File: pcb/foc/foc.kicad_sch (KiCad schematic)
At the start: 38 parts, among them J6 TB_MOTOR, J7 PH_2.0, Q4 BTN8982TA, Q5 BTN8982TA, Q6 BTN8982TA, U7 INA240A2PW, U8 INA240A2PW

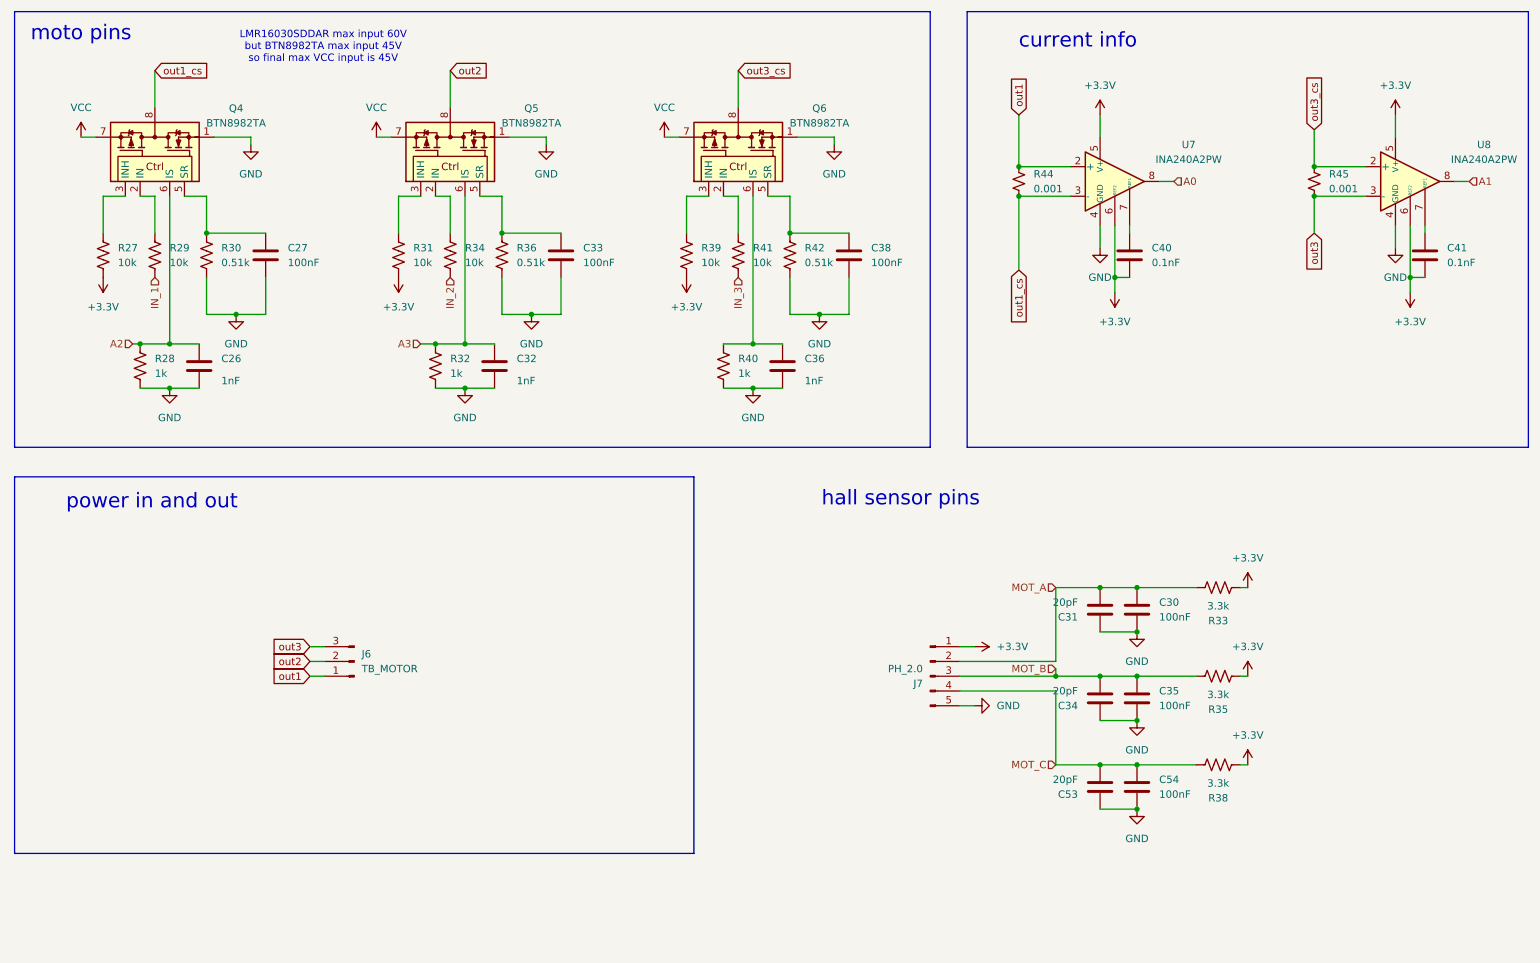
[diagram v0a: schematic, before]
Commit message: feat: update
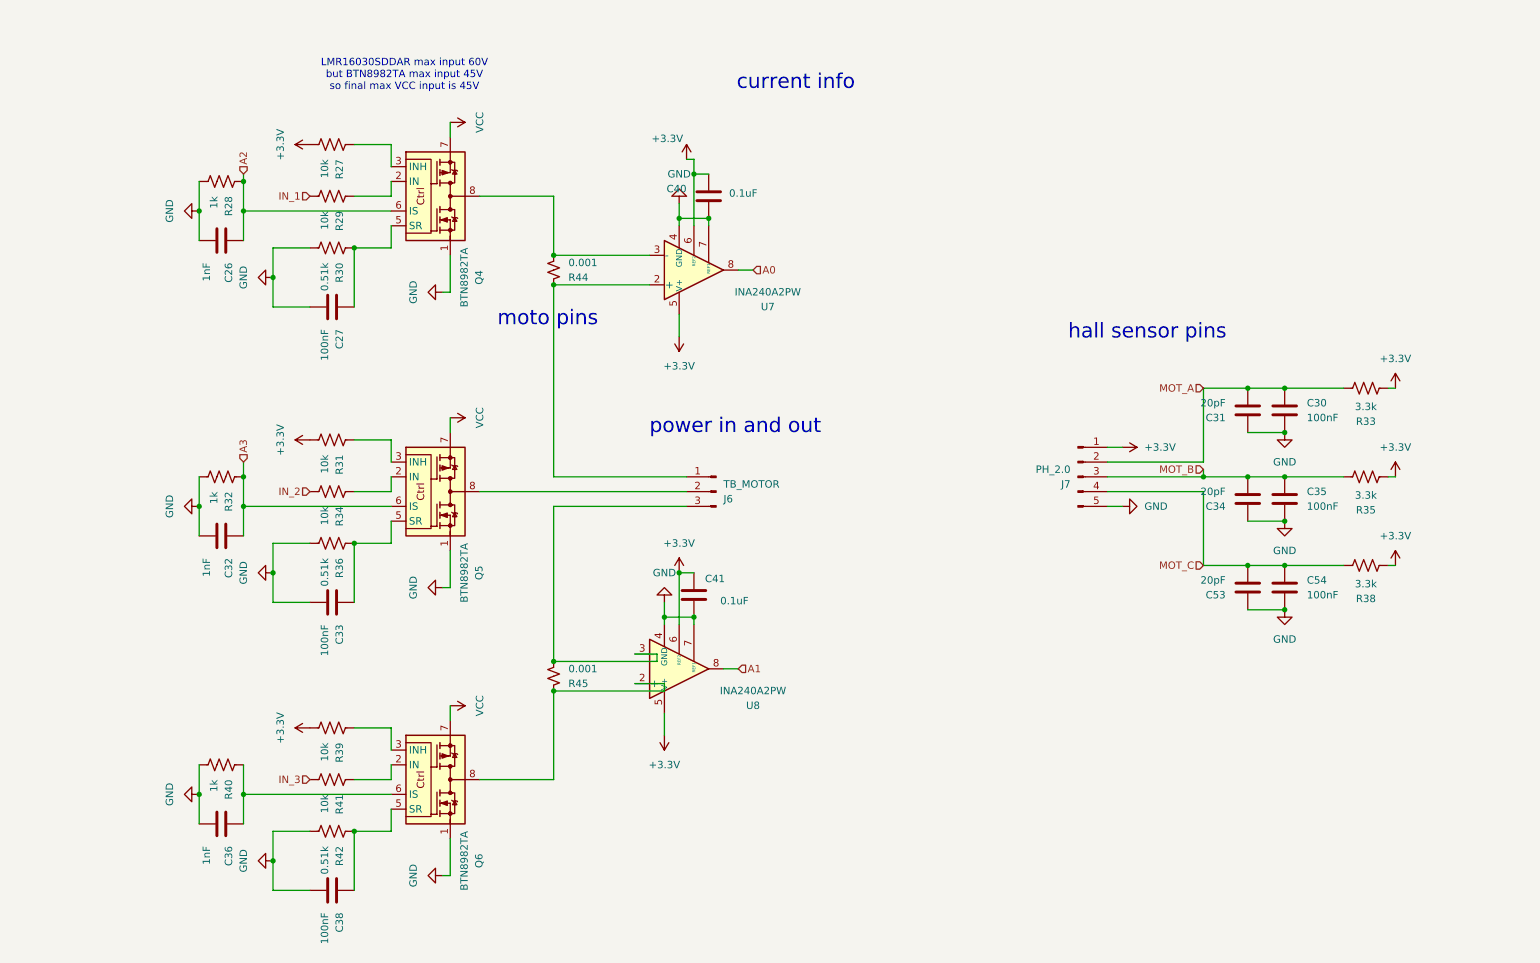
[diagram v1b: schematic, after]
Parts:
- C40, C41: value 0.1nF -> 0.1uF
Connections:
- net GND: now also C40.1, C41.1, U7.7 (REF1), U8.7 (REF1)
- net out1: no longer names the net of J6.1 (Pin_1), R44.1, U7.2 (+)
- net out1_cs: no longer names the net of Q4.4, Q4.8, R44.2, U7.3 (-)
- net out2: no longer names the net of J6.2 (Pin_2), Q5.4, Q5.8
- net out3: no longer names the net of J6.3 (Pin_3), R45.2, U8.3 (-)
- net out3_cs: no longer names the net of Q6.4, Q6.8, R45.1, U8.2 (+)
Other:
- moved on the sheet: C26, C27, C30, C31, C32, C33, C34, C35, C36, C38, C40, C41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
